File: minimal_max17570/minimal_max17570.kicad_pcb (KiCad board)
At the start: 4 copper layers, 15.2 x 12.7 mm, 11 parts, among them U1 MAX17570FATA+

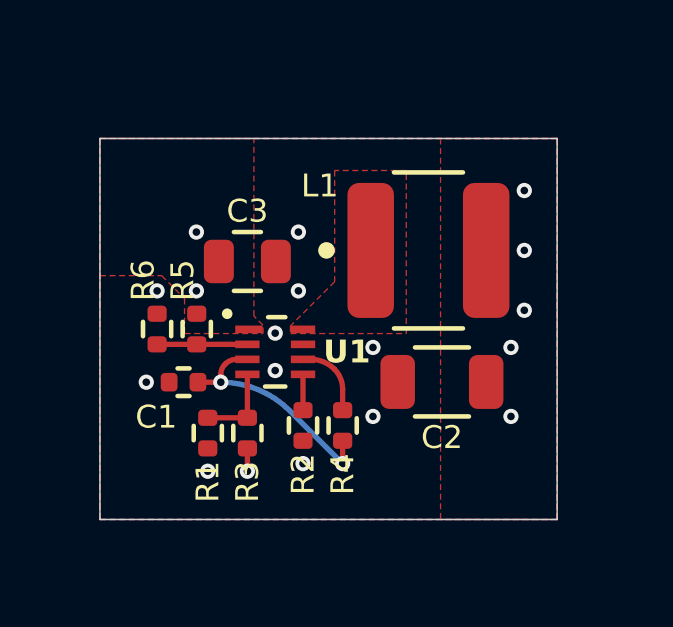
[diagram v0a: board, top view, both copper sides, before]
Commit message: backup
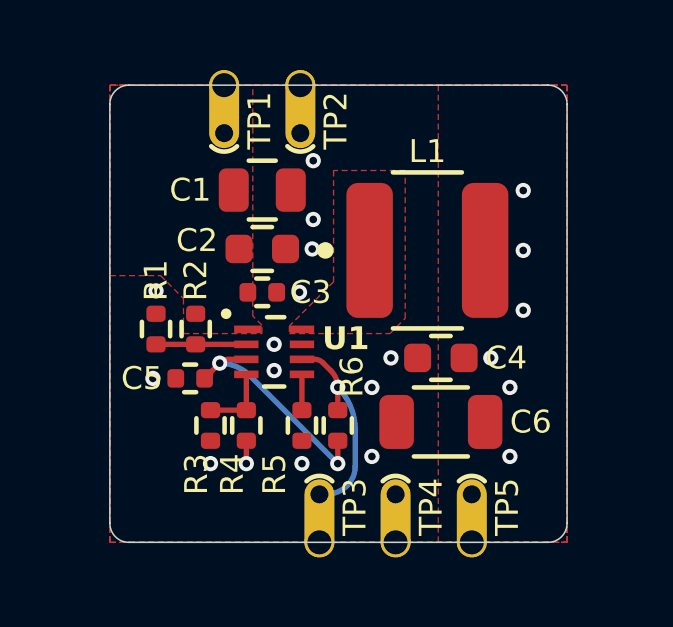
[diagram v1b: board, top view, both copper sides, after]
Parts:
- added C2: 100 nF, capacitor_footprints:C_0603_1608Metric, F.Cu at (146.9, 98.2)
- added C3: 220 pF, capacitor_footprints:C_0402_1005Metric, F.Cu at (146.9, 99.6)
- added C4: 100 nF, capacitor_footprints:C_0603_1608Metric, F.Cu at (152.8, 101.8)
- added TP1: TestPoint, test_point_footprints:TestPoint_THTPad_Castelated, F.Cu at (145.6, 92.7)
- added TP2: TestPoint, test_point_footprints:TestPoint_THTPad_Castelated, F.Cu at (148.2, 92.7)
- added TP3: TestPoint, test_point_footprints:TestPoint_THTPad_Castelated, F.Cu at (148.8, 108.0)
- added TP4: TestPoint, test_point_footprints:TestPoint_THTPad_Castelated, F.Cu at (151.3, 108.0)
- added TP5: TestPoint, test_point_footprints:TestPoint_THTPad_Castelated, F.Cu at (153.9, 108.0)
- moved C1 2.43 mm to (146.9, 96.2)
- moved C6 1.33 mm to (152.8, 103.9)
- moved R3 0.27 mm to (145.2, 104.1)
- moved R4 0.26 mm to (146.4, 104.1)
- moved C5 0.25 mm to (144.5, 102.5)
- moved R6 0.16 mm to (149.4, 104.1)
- renumbered C3 to C1, C1 to C5, C2 to C6, R6 to R1, R5 to R2, R1 to R3, R3 to R4, R2 to R5, R4 to R6
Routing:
- net /~{RESET}: track 2.56 -> 6.96 mm, vias 0 -> 1
- net GND: vias 10 -> 13
- net /VOUT: vias 6 -> 7
- net /VIN: vias 2 -> 0
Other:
- board size 15.2 x 12.7 mm -> 15.2 x 15.2 mm

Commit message: backup
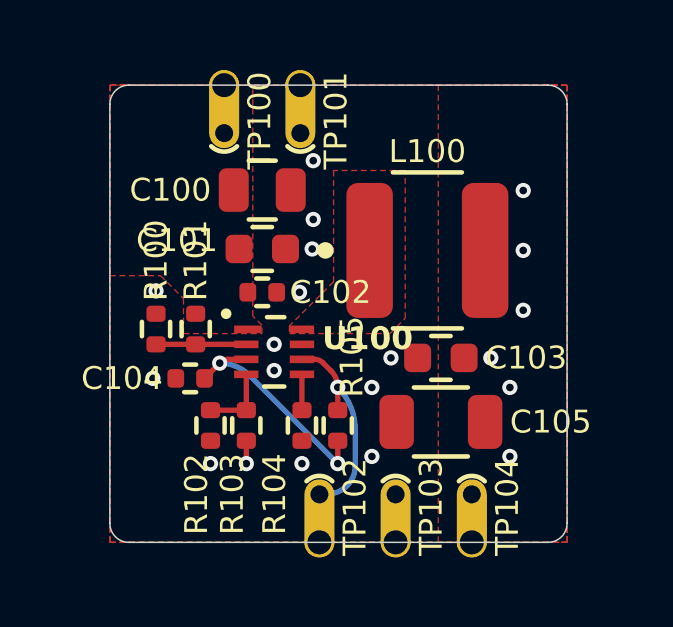
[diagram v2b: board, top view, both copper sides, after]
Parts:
- renumbered C1 to C100, C2 to C101, C3 to C102, C4 to C103, C5 to C104, C6 to C105, L1 to L100, R1 to R100, R2 to R101, R3 to R102, R4 to R103, R5 to R104, R6 to R105, TP1 to TP100, TP2 to TP101, TP3 to TP102, TP4 to TP103, TP5 to TP104, U1 to U100
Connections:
- net /VIN renamed /MAX17570_VIN
- net /VOUT renamed /MAX17570_VOUT
- net /~{RESET} renamed /~{MAX17570_RESET}

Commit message: backup
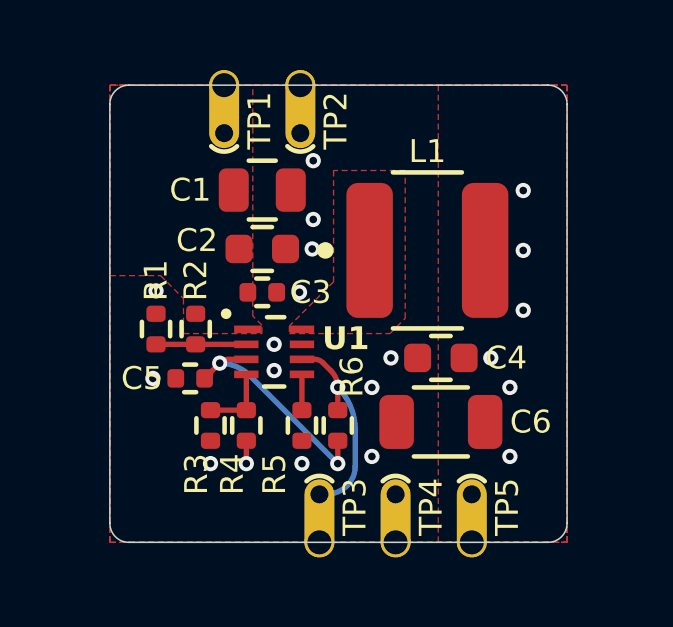
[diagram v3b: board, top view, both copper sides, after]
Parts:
- renumbered C100 to C1, C101 to C2, C102 to C3, C103 to C4, C104 to C5, C105 to C6, L100 to L1, R100 to R1, R101 to R2, R102 to R3, R103 to R4, R104 to R5, R105 to R6, TP100 to TP1, TP101 to TP2, TP102 to TP3, TP103 to TP4, TP104 to TP5, U100 to U1
